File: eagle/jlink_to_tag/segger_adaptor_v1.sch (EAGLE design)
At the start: 4 parts, among them U1 V_REG_LDOSMD

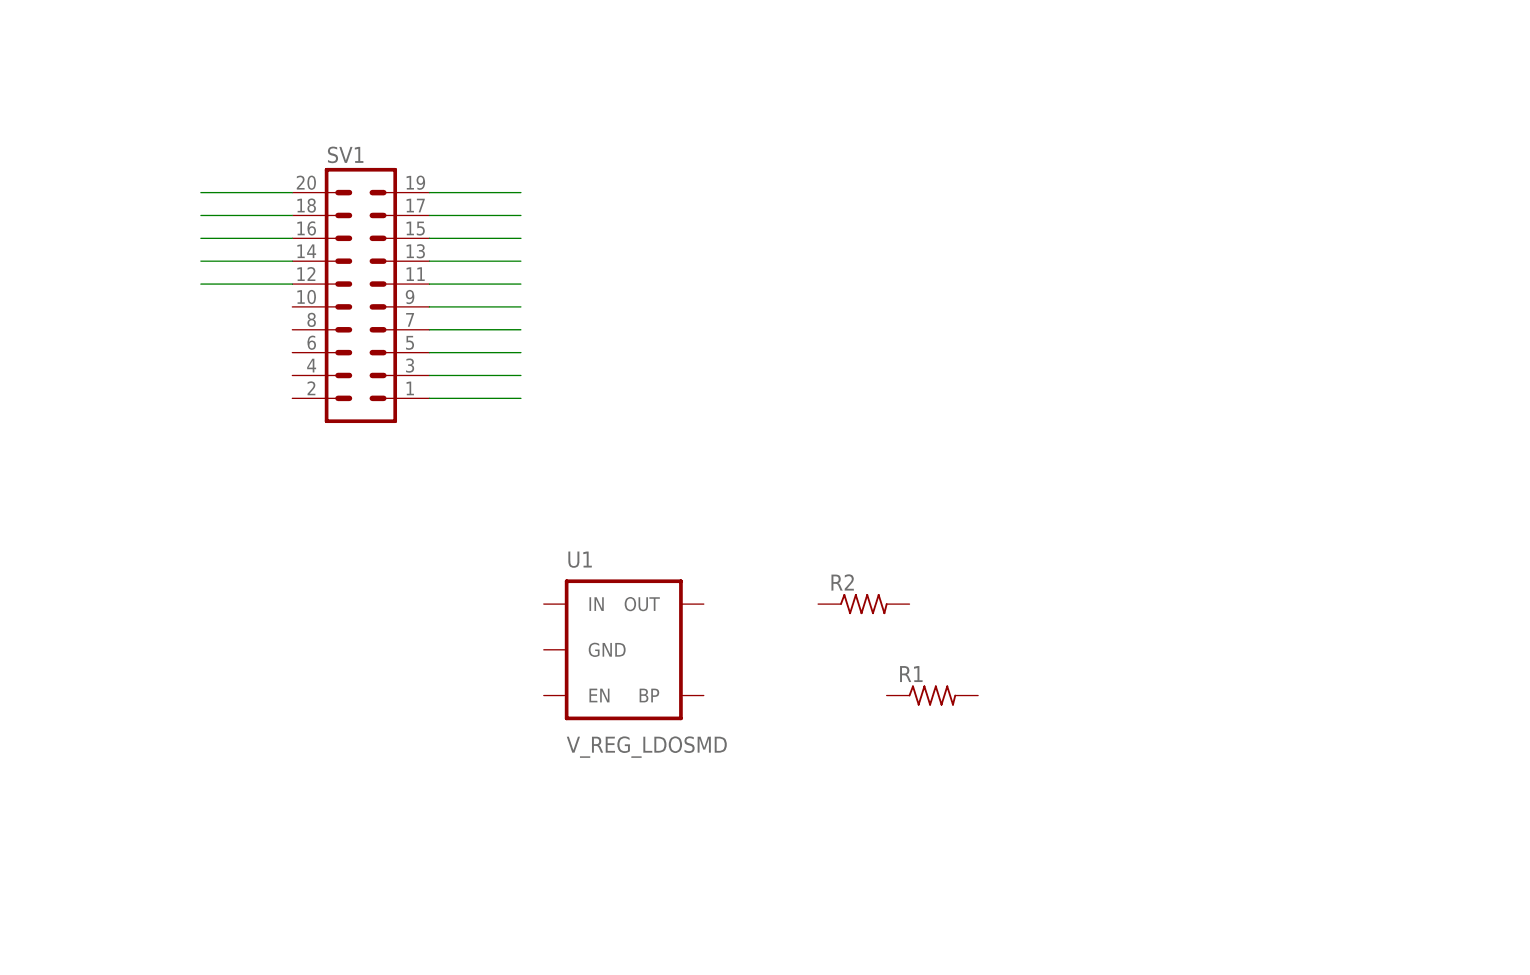
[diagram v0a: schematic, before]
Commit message: oops... wrong boards...
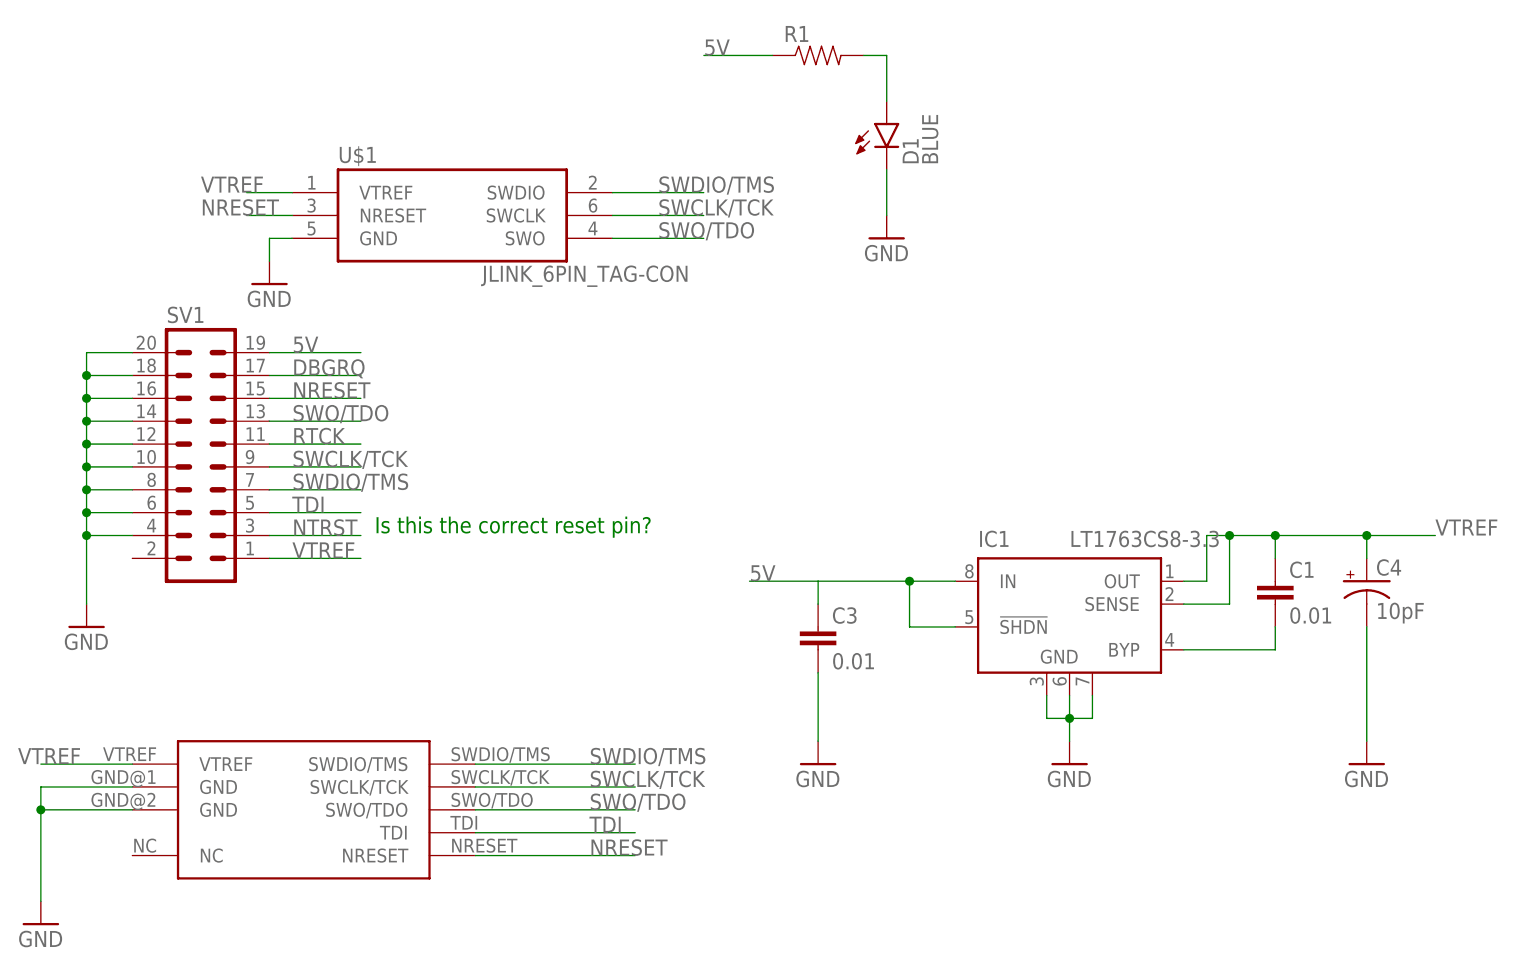
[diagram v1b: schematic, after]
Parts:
- removed R2: (no value), resistor:R-US_R0603
- removed U1: V_REG_LDOSMD, SparkFun-PowerIC:V_REG_LDOSMD
- added C1, C3: 0.01, resistor:C-EUC0603
- added C4: 10pF, SparkFun-Passives:CAP_POL1206
- added D1: BLUE, SparkFun-LED:LED-BLUE0603
- added IC1: LT1763CS8-3.3, linear-technology:LT1763CS8-3.3
- added U$1: JLINK_6PIN_TAG-CON, headers:JLINK_6PIN_TAG-CON
- added U$2: PINHD-2X3/0.050, headers:PINHD-2X3/0.050
- R1: device resistor:R-US_R0603 -> SparkFun-Passives:RESISTOR0402-RES
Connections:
- net N$2 renamed DBGRQ
- net N$5 renamed RTCK
- net N$9 renamed NTRST
- removed net N$1: SV1.19
- removed net N$10: SV1.1
- removed net N$11: SV1.20
- removed net N$12: SV1.18
- removed net N$13: SV1.16
- removed net N$14: SV1.14
- removed net N$15: SV1.12
- removed net N$6: SV1.9
- removed net N$7: SV1.7
- removed net N$8: SV1.5
- new net 5V: C3.1, IC1.!SHDN, IC1.IN, R1.1, SV1.19
- new net GND: C3.2, C4.-, D1.C, IC1.GND@1, IC1.GND@2, IC1.GND@3, SV1.10, SV1.12, SV1.14, SV1.16, SV1.18, SV1.20, SV1.4, SV1.6, SV1.8, U$1.GND, U$2.GND@1, U$2.GND@2
- new net NRESET: SV1.15, U$1.NRESET, U$2.NRESET
- new net SWCLK/TCK: SV1.9, U$1.SWCLK, U$2.SWCLK/TCK
- new net SWDIO/TMS: SV1.7, U$1.SWDIO, U$2.SWDIO/TMS
- new net SWO/TDO: SV1.13, U$1.SWO, U$2.SWO/TDO
- new net TDI: SV1.5, U$2.TDI
- new net VTREF: C1.1, C4.+, IC1.OUT, IC1.SENSE, SV1.1, U$1.VTREF, U$2.VTREF
- net N$3: now also D1.A, R1.2; no longer SV1.15
- net N$4: now also C1.2, IC1.BYP; no longer SV1.13
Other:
- note added: "Is this the correct reset pin?"
- moved on the sheet: R1, SV1
